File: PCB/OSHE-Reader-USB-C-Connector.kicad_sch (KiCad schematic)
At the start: 4 parts, among them J3 USB_C_Receptacle_PowerOnly_24P

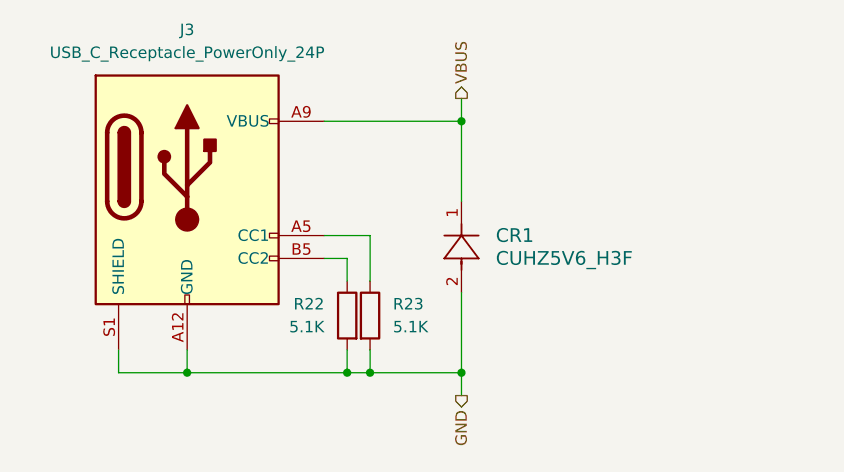
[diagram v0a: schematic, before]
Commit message: Did a bunch of work with final preparations of the schematic for pcb routing
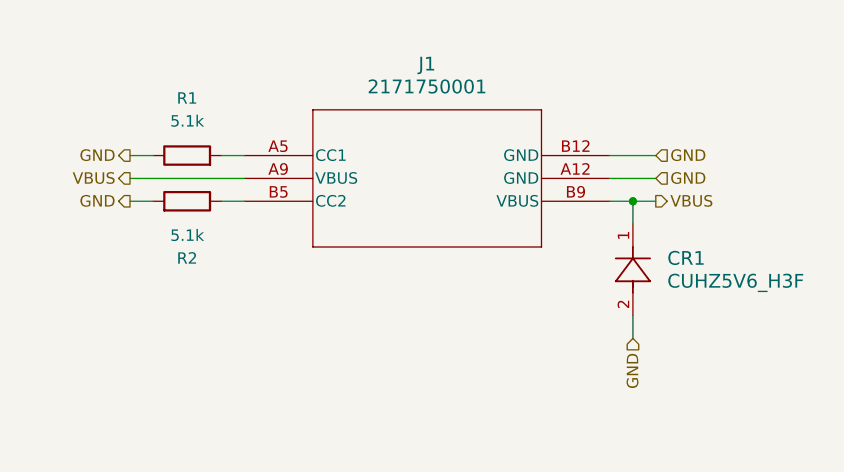
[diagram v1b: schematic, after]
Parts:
- removed J3: USB_C_Receptacle_PowerOnly_24P, USB4125_GF_A:CONN6_USB4125_GCT, symbol Connector:USB_C_Receptacle_PowerOnly_24P
- removed R22, R23: 5.1K, Resistor_SMD:R_1206_3216Metric, symbol Device:R
- added J1: 2171750001, 2171750001_MOL, symbol 2171750001:2171750001
- added R1, R2: 5.1k, Resistor_SMD:R_1206_3216Metric, symbol Device:R
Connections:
- net GND: now also J1.A12 (GND), J1.B12 (GND), R1.1, R2.2
- net VBUS: now also J1.A9 (VBUS), J1.B9 (VBUS)
- new net: J1.A5 (CC1), R1.2
- new net: J1.B5 (CC2), R2.1
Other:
- moved on the sheet: CR1
